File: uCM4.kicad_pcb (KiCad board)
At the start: 2 copper layers, 55 x 48 mm, 77 parts, among them IC1 MAX17048G+, J10 USB_C_Receptacle, J12 Conn_02x08_Odd_Even, J13 Conn_02x07_Odd_Even, J2 Micro_SD_Card_Det, J4 Conn_01x04, J5 DummyJ, J6 DummyJ, J8 Camera 0, J9 Camera 1, Q2 AO3401A, SW1 SW_DIP_x01, SW3 SW_Push, SW4 SW_SPDT, U1 BNO055, U18 RT9742GGJ5, U2 SN74LVC1G07DBVR, U3 TPD4EUSB30DQAR, U4 TPS61022, U6 TP4057

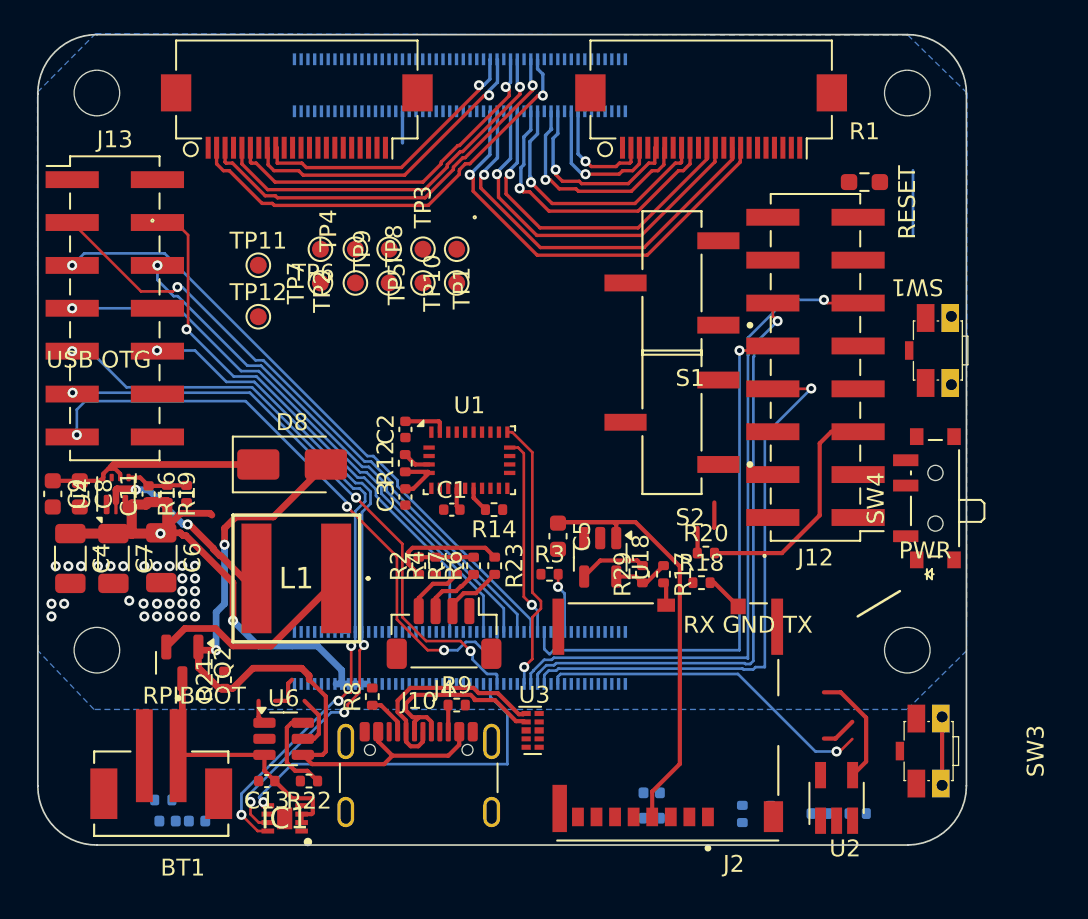
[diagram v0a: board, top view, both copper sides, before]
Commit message: Routing
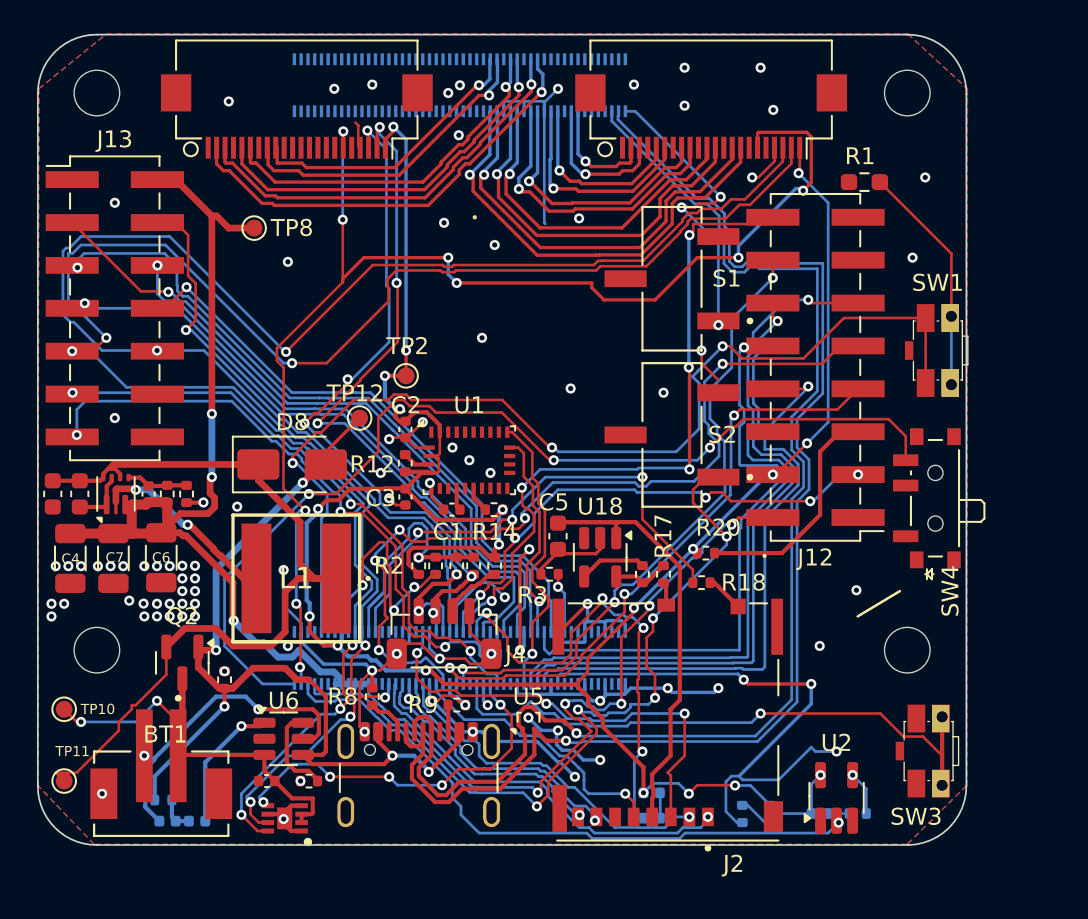
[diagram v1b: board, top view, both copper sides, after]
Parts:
- removed TP1, TP3, TP4, TP5, TP6, TP7, TP9: TestPoint, TestPoint:TestPoint_Pad_D1.0mm
- removed U3: TPD4EUSB30DQAR, Package_SON:USON-10_2.5x1.0mm_P0.5mm
- added U5: TPD2EUSB30, Package_TO_SOT_SMD:Texas_DRT-3, F.Cu at (150.0, 125.8)
- moved TP10 34.3 mm to (122.5, 125.0)
- moved TP11 32.6 mm to (122.5, 129.2)
- moved TP2 9.05 mm to (142.8, 105.2)
- moved TP8 8.63 mm to (133.8, 96.5)
- moved TP12 8.49 mm to (140.0, 107.8)
- moved S2 0.75 mm to (158.5, 108.8)
- moved S1 0.25 mm to (158.5, 99.5)
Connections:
- Module1 pad 37: /ENV_SEL -> unconnected-(Module1A-GPIO7-Pad37)
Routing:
- net GND: track 1.88 -> 137.5 mm, vias 29 -> 95
- net +3V3: track 14.8 -> 141.7 mm, vias 0 -> 19
- net /CAM_GPIO: track 0.00 -> 77.1 mm, vias 0 -> 9
- net /USB_P: track 11.8 -> 78.7 mm, vias 0 -> 1
- net /USB_N: track 13.0 -> 78.2 mm, vias 0 -> 1
- net +5V: track 32.8 -> 97.9 mm, vias 2 -> 8
- net /SCL0: track 40.2 -> 102.7 mm, vias 4 -> 5
- net /RESET: track 0.00 -> 62.0 mm, vias 0 -> 3
- net /SDA0: track 45.2 -> 107.0 mm, vias 4 -> 6
- net Net-(Module1A-Global_EN): track 3.85 -> 59.3 mm, vias 0 -> 3
- net /TXD0: track 0.00 -> 50.3 mm, vias 0 -> 5
- net Net-(Module1A-nRPIBOOT): track 0.00 -> 46.5 mm, vias 0 -> 5
- net /SPI6_CE1_N: track 0.00 -> 41.0 mm, vias 0 -> 5
- net /SCL1: track 3.60 -> 42.4 mm, vias 0 -> 5
- net /SPI6_CE0_N: track 0.00 -> 37.6 mm, vias 0 -> 3
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- added copper zone on F.Cu, net GND
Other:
- board text removed: "ACT"
- board text removed: "PWR"
- board text removed: "RESET"
- board text removed: "RPIBOOT"
- board text removed: "RX GND TX"
- board text removed: "USB OTG"
